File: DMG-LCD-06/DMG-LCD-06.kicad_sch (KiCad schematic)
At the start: 46 parts, among them J1 Wire, J2 Wire, J3 Wire, J4 Wire, J5 Wire, Q1 2SA933SR, SW1 Left, SW2 Up, SW3 Down, SW4 Right, SW5 Select, SW6 Start, SW7 B, SW8 A, U1 IR3E02, U2 LH5076, U3 LH5077

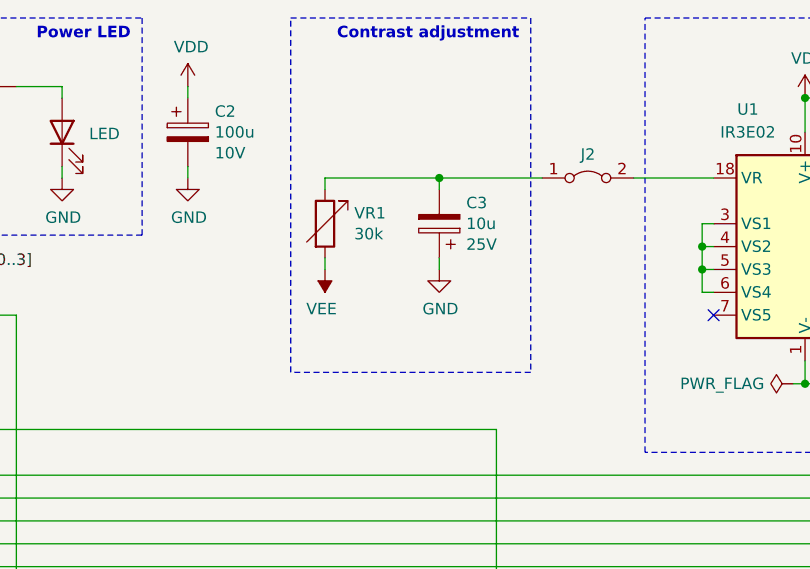
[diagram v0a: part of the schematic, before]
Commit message: Tidy up potentiometer symbols, add contrast pot symbols
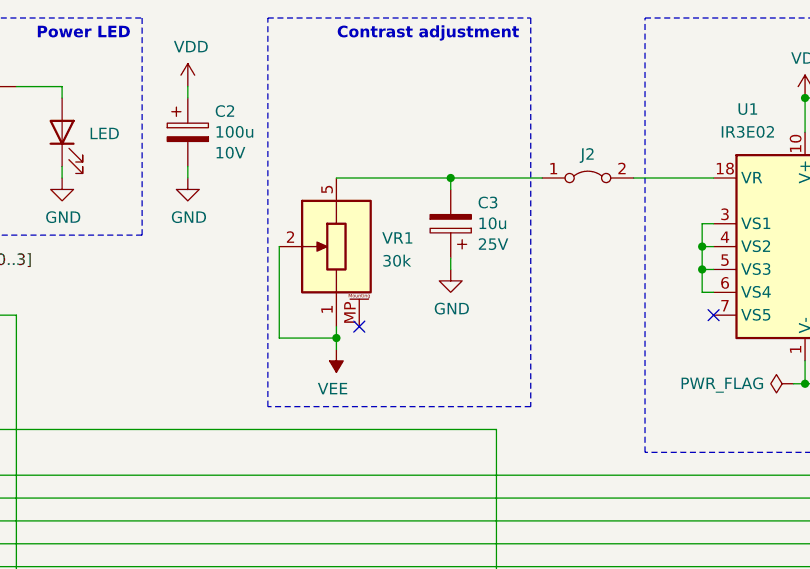
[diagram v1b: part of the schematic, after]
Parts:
- VR1: symbol Device:R_Variable -> Gekkio_Device_Specialized:R_Potentiometer_GameBoy_Contrast_DMG
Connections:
- net VEE: now also VR1.1 (4)
- net at C3.2, J2.1 (A): now also VR1.5; no longer VR1.1
- no-connect marks 2 -> 3
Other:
- moved on the sheet: C3
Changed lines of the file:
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@@
   (junction (at 222.25 20.32) (diameter 0) (color 0 0 0 0)
   )
-  (junction (at 109.22 31.75) (diameter 0) (color 0 0 0 0)
-  )
   (junction (at 149.86 22.86) (diameter 0) (color 0 0 0 0)
   )
@@
   (junction (at 199.39 20.32) (diameter 0) (color 0 0 0 0)
   )
+  (junction (at 110.49 31.75) (diameter 0) (color 0 0 0 0)
+  )
   (junction (at 115.57 95.25) (diameter 0) (color 0 0 0 0)
   )
@@
   (junction (at 210.82 36.83) (diameter 0) (color 0 0 0 0)
   )
+  (junction (at 97.79 49.53) (diameter 0) (color 0 0 0 0)
+  )
   (junction (at 181.61 20.32) (diameter 0) (color 0 0 0 0)
   )
@@
   (junction (at 228.6 157.48) (diameter 0) (color 0 0 0 0)
   )
+  (no_connect (at 100.33 48.26))
   (no_connect (at 139.7 46.99))
   (no_connect (at 259.08 87.63))
@@
     (stroke (width 0) (type default))
   )
-  (wire (pts (xy 96.52 33.02) (xy 96.52 31.75))
-    (stroke (width 0) (type default))
-  )
   (wire (pts (xy 213.36 36.83) (xy 213.36 34.29))
     (stroke (width 0) (type default))
@@
     (stroke (width 0) (type default))
   )
-  (wire (pts (xy 96.52 41.91) (xy 96.52 40.64))
+  (wire (pts (xy 97.79 48.26) (xy 97.79 49.53))
     (stroke (width 0) (type default))
   )
@@
     (stroke (width 0) (type default))
   )
+  (wire (pts (xy 91.44 49.53) (xy 97.79 49.53))
+    (stroke (width 0) (type default))
+  )
   (wire (pts (xy 49.53 59.69) (xy 115.57 59.69))
     (stroke (width 0) (type default))
@@
   )
   (wire (pts (xy 152.4 92.71) (xy 133.35 92.71))
+    (stroke (width 0) (type default))
+  )
+  (wire (pts (xy 97.79 49.53) (xy 97.79 50.8))
     (stroke (width 0) (type default))
   )
@@
     (stroke (width 0) (type default))
   )
-  (wire (pts (xy 96.52 31.75) (xy 109.22 31.75))
-    (stroke (width 0) (type default))
-  )
   (wire (pts (xy 266.7 100.33) (xy 266.7 95.25))
     (stroke (width 0) (type default))
@@
     (stroke (width 0) (type default))
   )
+  (wire (pts (xy 91.44 39.37) (xy 91.44 49.53))
+    (stroke (width 0) (type default))
+  )
   (wire (pts (xy 123.19 179.07) (xy 123.19 166.37))
     (stroke (width 0) (type default))
@@
     (stroke (width 0) (type default))
   )
+  (wire (pts (xy 97.79 31.75) (xy 110.49 31.75))
+    (stroke (width 0) (type default))
+  )
   (wire (pts (xy 22.86 46.99) (xy 62.23 46.99))
     (stroke (width 0) (type default))
@@
     (stroke (width 0) (type default))
   )
-  (wire (pts (xy 109.22 33.02) (xy 109.22 31.75))
+  (wire (pts (xy 110.49 33.02) (xy 110.49 31.75))
     (stroke (width 0) (type default))
   )
@@
     (stroke (width 0) (type dash))
   )
-  (wire (pts (xy 120.65 31.75) (xy 109.22 31.75))
+  (wire (pts (xy 120.65 31.75) (xy 110.49 31.75))
     (stroke (width 0) (type default))
   )
@@
     (stroke (width 0) (type default))
   )
-  (wire (pts (xy 109.22 41.91) (xy 109.22 40.64))
+  (wire (pts (xy 110.49 41.91) (xy 110.49 40.64))
     (stroke (width 0) (type default))
   )
@@
     (fill (type none))
   )
-  (rectangle (start 92.71 13.97) (end 119.38 53.34)
+  (rectangle (start 90.17 13.97) (end 119.38 57.15)
     (stroke (width 0) (type dash))
     (fill (type none))
@@
     )
   )
-  (symbol (lib_id "Device:R_Variable") (at 96.52 36.83 0) (unit 1)
-    (in_bom yes) (on_board yes) (dnp no)
-    (property "Reference" "VR1" (at 99.7712 35.6616 0)
+  (symbol (lib_id "Gekkio_Device_Specialized:R_Potentiometer_GameBoy_Contrast_DMG") (at 97.79 39.37 0) (unit 1)
+    (in_bom yes) (on_board yes) (dnp no) (fields_autoplaced)
+    (property "Reference" "VR1" (at 102.87 38.4556 0)
       (effects (font (size 1.27 1.27)) (justify left))
     )
-    (property "Value" "30k" (at 99.7712 37.973 0)
+    (property "Value" "30k" (at 102.87 40.9956 0)
       (effects (font (size 1.27 1.27)) (justify left))
     )
-    (property "Footprint" "" (at 94.742 36.83 90)
-      (effects (font (size 1.27 1.27)) hide)
-    )
-    (property "Datasheet" "~" (at 96.52 36.83 0)
+    (property "Footprint" "" (at 99.695 33.02 90)
+      (effects (font (size 1.27 1.27)) hide)
+    )
+    (property "Datasheet" "~" (at 99.695 33.02 90)
       (effects (font (size 1.27 1.27)) hide)
     )
     (pin "1")
     (pin "2")
+    (pin "5")
+    (pin "MP")
     (instances
       (project "DMG-LCD-06"
@@
     )
   )
-  (symbol (lib_id "power:VEE") (at 96.52 41.91 180) (unit 1)
+  (symbol (lib_id "power:VEE") (at 97.79 50.8 180) (unit 1)
     (in_bom yes) (on_board yes) (dnp no)
-    (property "Reference" "#PWR0101" (at 96.52 38.1 0)
-      (effects (font (size 1.27 1.27)) hide)
-    )
-    (property "Value" "VEE" (at 96.139 46.3042 0)
+    (property "Reference" "#PWR0101" (at 97.79 46.99 0)
+      (effects (font (size 1.27 1.27)) hide)
+    )
+    (property "Value" "VEE" (at 97.409 55.1942 0)
       (effects (font (size 1.27 1.27)))
     )
-    (property "Footprint" "" (at 96.52 41.91 0)
-      (effects (font (size 1.27 1.27)) hide)
-    )
-    (property "Datasheet" "" (at 96.52 41.91 0)
+    (property "Footprint" "" (at 97.79 50.8 0)
+      (effects (font (size 1.27 1.27)) hide)
+    )
+    (property "Datasheet" "" (at 97.79 50.8 0)
       (effects (font (size 1.27 1.27)) hide)
     )
@@
     )
   )
-  (symbol (lib_id "Device:C_Polarized") (at 109.22 36.83 180) (unit 1)
+  (symbol (lib_id "Device:C_Polarized") (at 110.49 36.83 180) (unit 1)
     (in_bom yes) (on_board yes) (dnp no)
-    (property "Reference" "C3" (at 112.2172 34.5186 0)
+    (property "Reference" "C3" (at 113.4872 34.5186 0)
       (effects (font (size 1.27 1.27)) (justify right))
     )
-    (property "Value" "10u" (at 112.2172 36.83 0)
+    (property "Value" "10u" (at 113.4872 36.83 0)
       (effects (font (size 1.27 1.27)) (justify right))
     )
-    (property "Footprint" "" (at 108.2548 33.02 0)
-      (effects (font (size 1.27 1.27)) hide)
-    )
-    (property "Datasheet" "~" (at 109.22 36.83 0)
-      (effects (font (size 1.27 1.27)) hide)
-    )
-    (property "Rating" "25V" (at 112.2172 39.1414 0)
+    (property "Footprint" "" (at 109.5248 33.02 0)
+      (effects (font (size 1.27 1.27)) hide)
+    )
+    (property "Datasheet" "~" (at 110.49 36.83 0)
+      (effects (font (size 1.27 1.27)) hide)
+    )
+    (property "Rating" "25V" (at 113.4872 39.1414 0)
       (effects (font (size 1.27 1.27)) (justify right))
     )
@@
     )
   )
-  (symbol (lib_id "power:GND") (at 109.22 41.91 0) (unit 1)
+  (symbol (lib_id "power:GND") (at 110.49 41.91 0) (unit 1)
     (in_bom yes) (on_board yes) (dnp no)
-    (property "Reference" "#PWR0106" (at 109.22 48.26 0)
-      (effects (font (size 1.27 1.27)) hide)
-    )
-    (property "Value" "GND" (at 109.347 46.3042 0)
+    (property "Reference" "#PWR0106" (at 110.49 48.26 0)
+      (effects (font (size 1.27 1.27)) hide)
+    )
+    (property "Value" "GND" (at 110.617 46.3042 0)
       (effects (font (size 1.27 1.27)))
     )
-    (property "Footprint" "" (at 109.22 41.91 0)
-      (effects (font (size 1.27 1.27)) hide)
-    )
-    (property "Datasheet" "" (at 109.22 41.91 0)
-      (effects (font (size 1.27 1.27)) hide)
-    )
+    (property "Footprint" "" (at 110.49 41.91 0)
+      (effects (font (size 1.27 1.27)) hide)
+    )
+    (property "Datasheet" "" (at 110.49 41.91 0)
+      (effects (font (size 1.27 1.27)) hide)
+    )
